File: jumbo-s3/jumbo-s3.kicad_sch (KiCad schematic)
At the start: 26 parts, among them J1 GPIO, J2 DEBUG, U1 ESP32-S3, U2 APS12808L-3OBM-BA, Y1 40MHz 10ppm

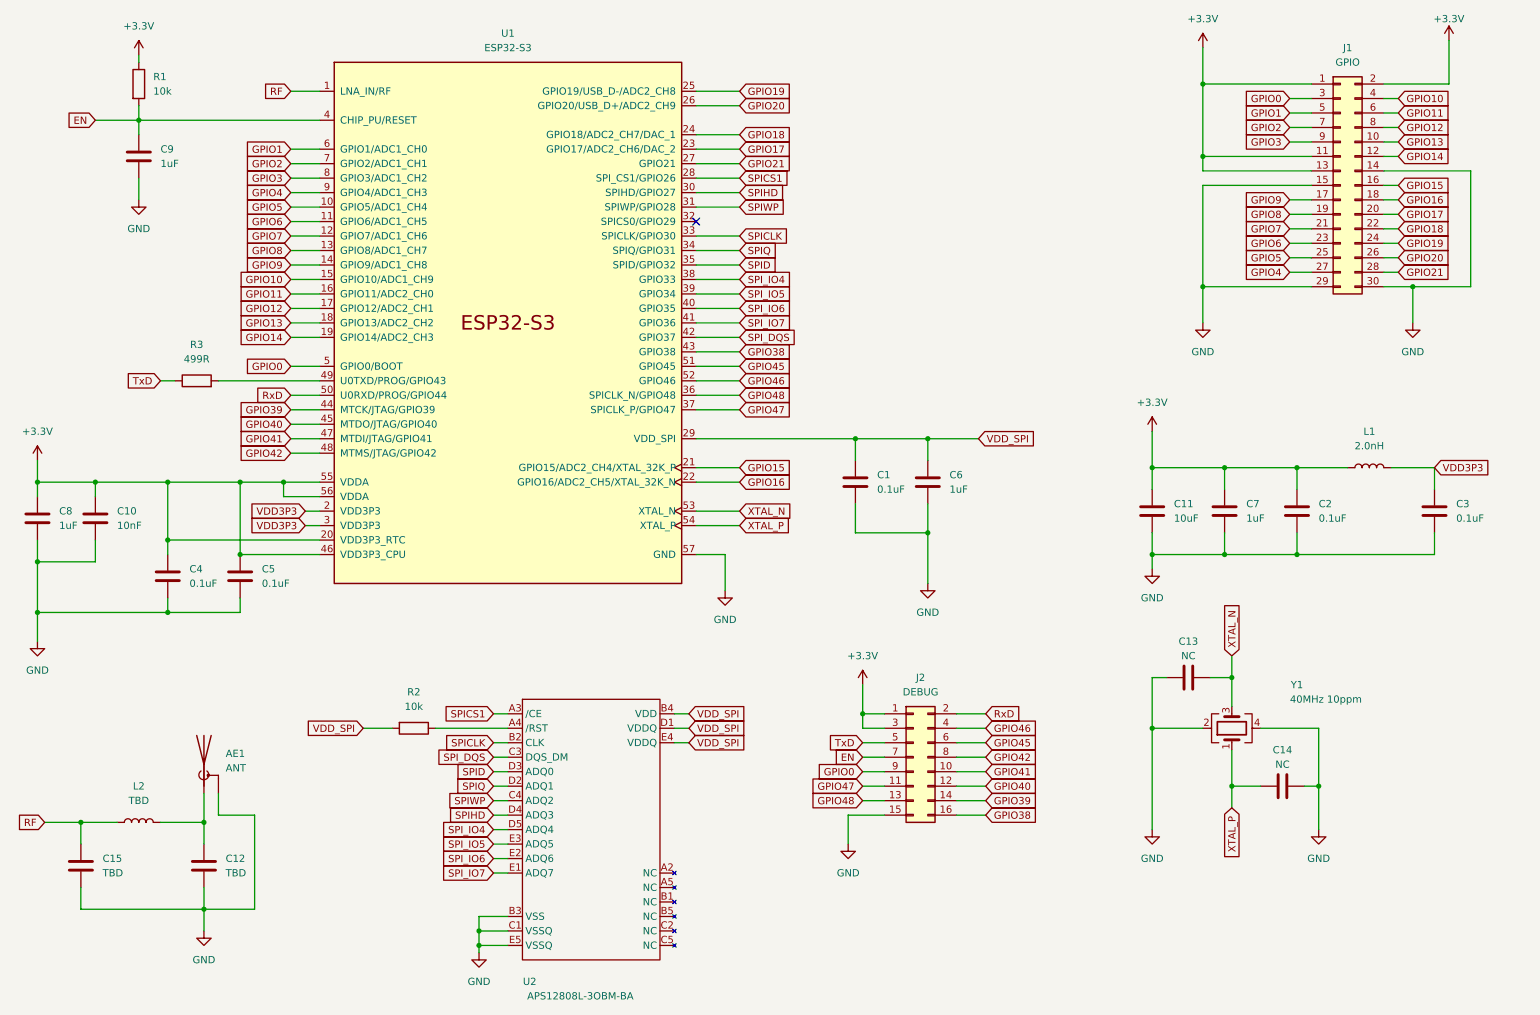
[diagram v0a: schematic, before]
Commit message: Rev 2.1: unify headers
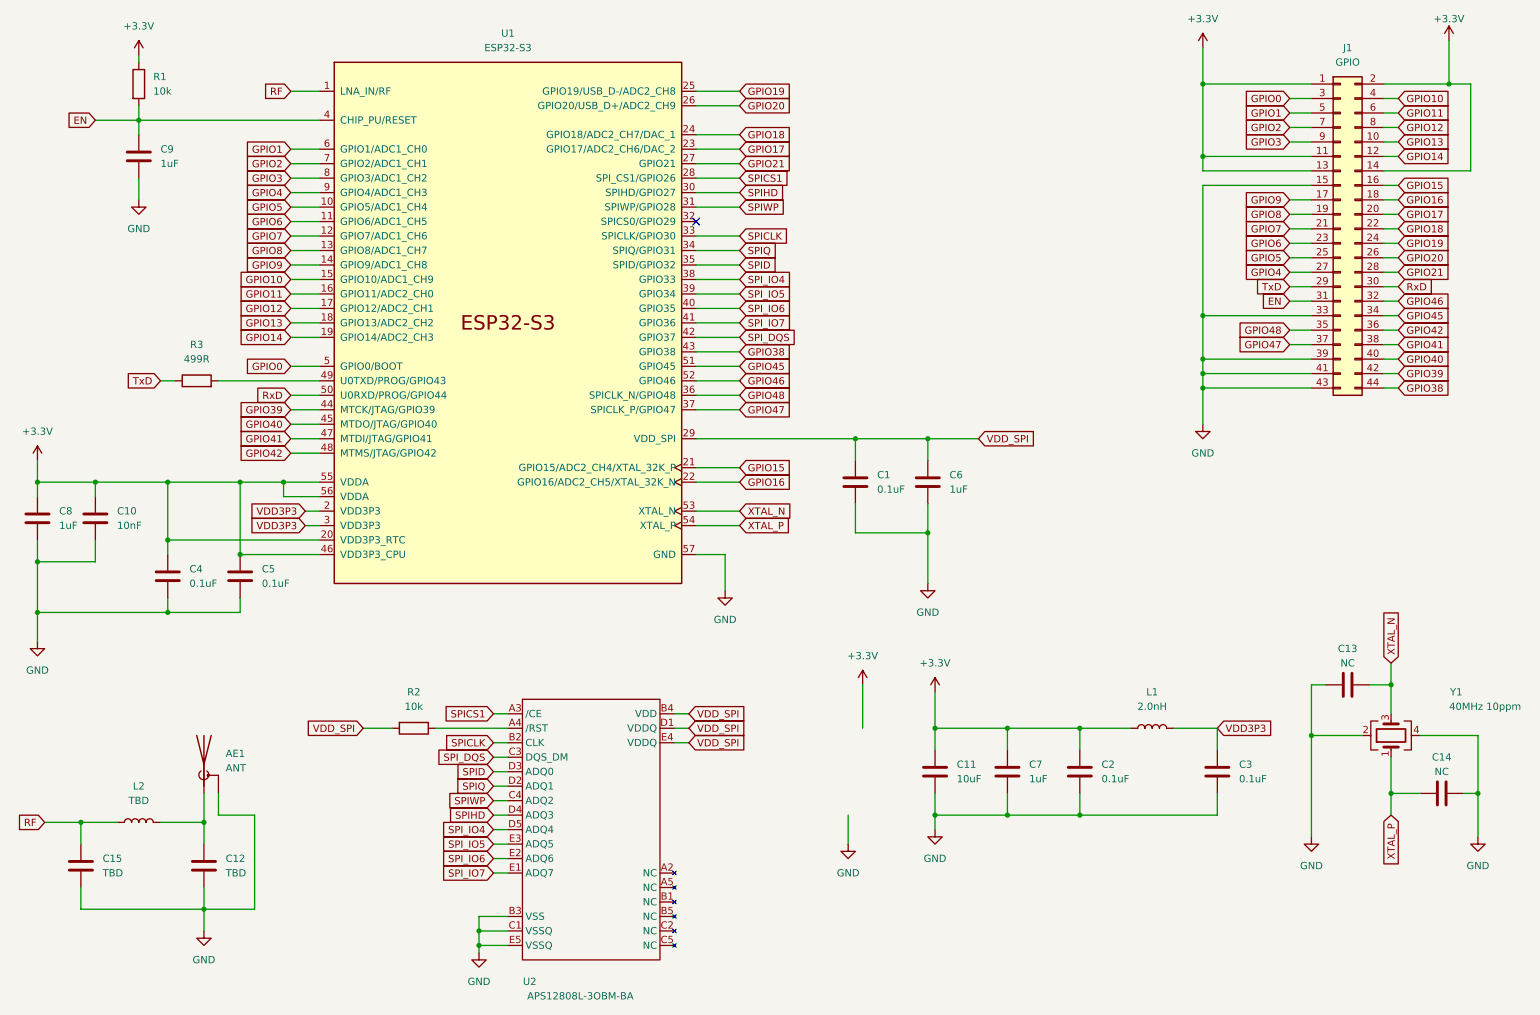
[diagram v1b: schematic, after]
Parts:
- removed J1: GPIO, Connector_PinHeader_1.27mm:PinHeader_2x15_P1.27mm_Vertical_SMD, symbol Connector_Generic:Conn_02x15_Odd_Even
- removed J2: DEBUG, Connector_PinHeader_1.27mm:PinHeader_2x08_P1.27mm_Vertical_SMD, symbol Connector_Generic:Conn_02x08_Odd_Even
- added J1: GPIO, Connector_PinHeader_1.27mm:PinHeader_2x22_P1.27mm_Vertical_SMD, symbol Connector_Generic:Conn_02x22_Odd_Even
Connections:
- net +3.3V: now also J1.1 (Pin_1), J1.11 (Pin_11), J1.13 (Pin_13), J1.14 (Pin_14), J1.2 (Pin_2)
- net EN: now also J1.31 (Pin_31)
- net GND: now also J1.15 (Pin_15), J1.33 (Pin_33), J1.39 (Pin_39), J1.41 (Pin_41), J1.43 (Pin_43)
- net GPIO0: now also J1.3 (Pin_3)
- net GPIO1: now also J1.5 (Pin_5)
- net GPIO10: now also J1.4 (Pin_4)
- net GPIO11: now also J1.6 (Pin_6)
- net GPIO12: now also J1.8 (Pin_8)
- net GPIO13: now also J1.10 (Pin_10)
- net GPIO14: now also J1.12 (Pin_12)
- net GPIO15: now also J1.16 (Pin_16)
- net GPIO16: now also J1.18 (Pin_18)
- net GPIO17: now also J1.20 (Pin_20)
- net GPIO18: now also J1.22 (Pin_22)
- net GPIO19: now also J1.24 (Pin_24)
- net GPIO2: now also J1.7 (Pin_7)
- net GPIO20: now also J1.26 (Pin_26)
- net GPIO21: now also J1.28 (Pin_28)
- net GPIO3: now also J1.9 (Pin_9)
- net GPIO38: now also J1.44 (Pin_44)
- net GPIO39: now also J1.42 (Pin_42)
- net GPIO4: now also J1.27 (Pin_27)
- net GPIO40: now also J1.40 (Pin_40)
- net GPIO41: now also J1.38 (Pin_38)
- net GPIO42: now also J1.36 (Pin_36)
- net GPIO45: now also J1.34 (Pin_34)
- net GPIO46: now also J1.32 (Pin_32)
- net GPIO47: now also J1.37 (Pin_37)
- net GPIO48: now also J1.35 (Pin_35)
- net GPIO5: now also J1.25 (Pin_25)
- net GPIO6: now also J1.23 (Pin_23)
- net GPIO7: now also J1.21 (Pin_21)
- net GPIO8: now also J1.19 (Pin_19)
- net GPIO9: now also J1.17 (Pin_17)
- net RxD: now also J1.30 (Pin_30)
- net TxD: now also J1.29 (Pin_29)
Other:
- moved on the sheet: C11, C13, C14, C2, C3, C7, L1, Y1
